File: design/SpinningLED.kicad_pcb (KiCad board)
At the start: 2 copper layers, 67.5 x 67.5 mm, 25 parts, among them IC1 4069, IC2 4017, P1 CONN_2, SW1 SW_PUSH

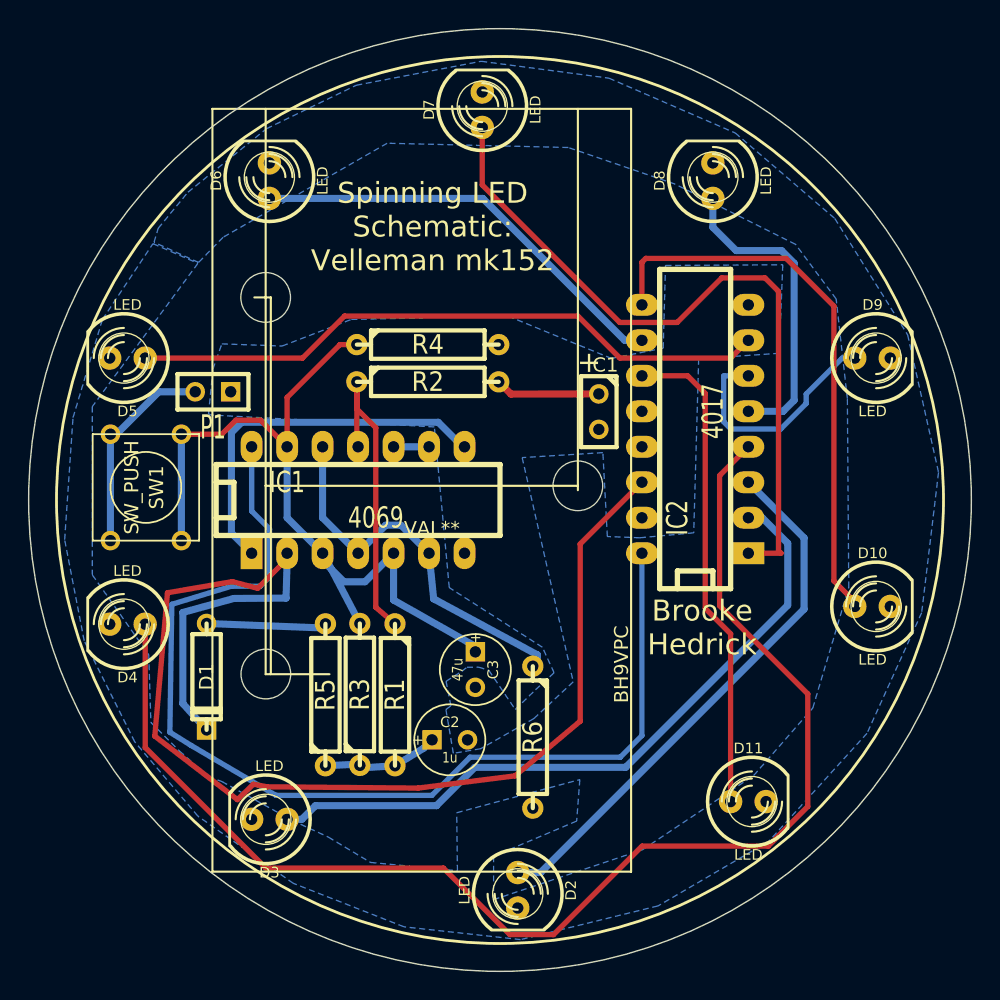
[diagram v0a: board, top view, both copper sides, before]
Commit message: SpinningLED v3
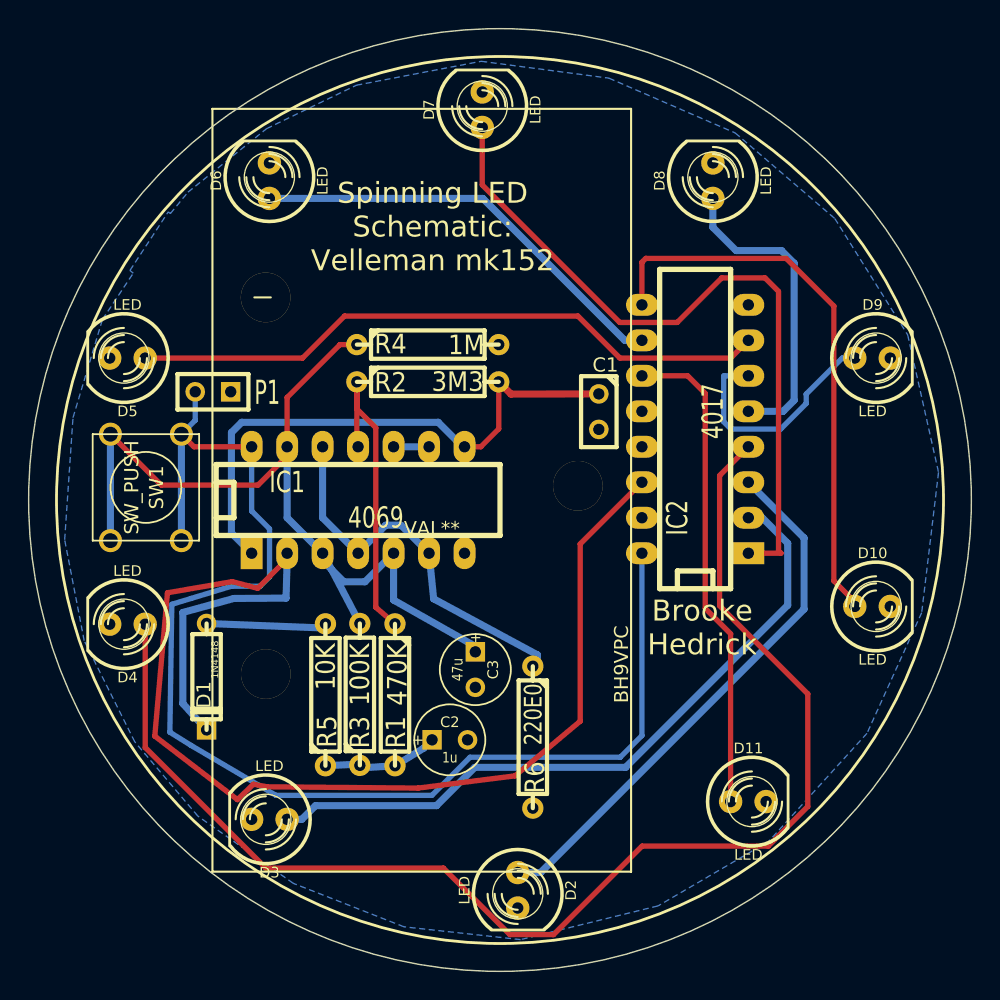
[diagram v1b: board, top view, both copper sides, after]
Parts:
- SW1: footprint SW_PUSH_SMALL -> SW_PUSH_SMALL_BTH
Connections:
- C1 pad 1: N-0000018 -> N-0000015
- C3 pad 1: N-0000023 -> +9V
- D10 pad 2: /ResToLEDs -> GND
- D11 pad 2: /ResToLEDs -> GND
- D2 pad 2: /ResToLEDs -> GND
- D3 pad 2: /ResToLEDs -> GND
- D4 pad 2: /ResToLEDs -> GND
- D5 pad 2: /ResToLEDs -> GND
- D6 pad 2: /ResToLEDs -> GND
- D7 pad 2: /ResToLEDs -> GND
- D8 pad 2: /ResToLEDs -> GND
- D9 pad 2: /ResToLEDs -> GND
- IC1 pad 1: N-0000017 -> N-0000015
- IC1 pad 13: N-0000023 -> +9V
- IC1 pad 3: N-0000023 -> +9V
- IC1 pad 5: N-0000023 -> +9V
- IC1 pad 8: N-0000017 -> N-0000015
- P1 pad 2: +9V -> VCC
- R2 pad 2: N-0000018 -> N-0000015
- R3 pad 2: N-0000023 -> +9V
- R4 pad 1: N-0000023 -> +9V
- R6 pad 2: /ResToLEDs -> GND
- SW1 pad 1: N-0000023 -> VCC
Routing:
- net N-0000023: track 58.4 -> 0.00 mm
- net +9V: track 14.9 -> 65.3 mm
- net N-0000015: track 0.00 -> 40.8 mm
- net N-0000017: track 27.0 -> 0.00 mm
- net VCC: track 76.3 -> 92.8 mm
- net N-0000018: track 7.53 -> 0.00 mm
- removed copper zone on B.Cu, net /ResToLEDs
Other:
- net class BigConnect added: clearance 0.254, trace_width 1.778, via_dia 0.889, via_drill 0.635
- board text added: "+9V-"
- board text added: "10n"
- board text removed: "+"
